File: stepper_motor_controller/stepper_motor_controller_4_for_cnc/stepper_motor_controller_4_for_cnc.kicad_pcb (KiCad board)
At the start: 2 copper layers, 31 parts, among them U1 74LS74, U11 LM317_TO-220, U3 74LS136

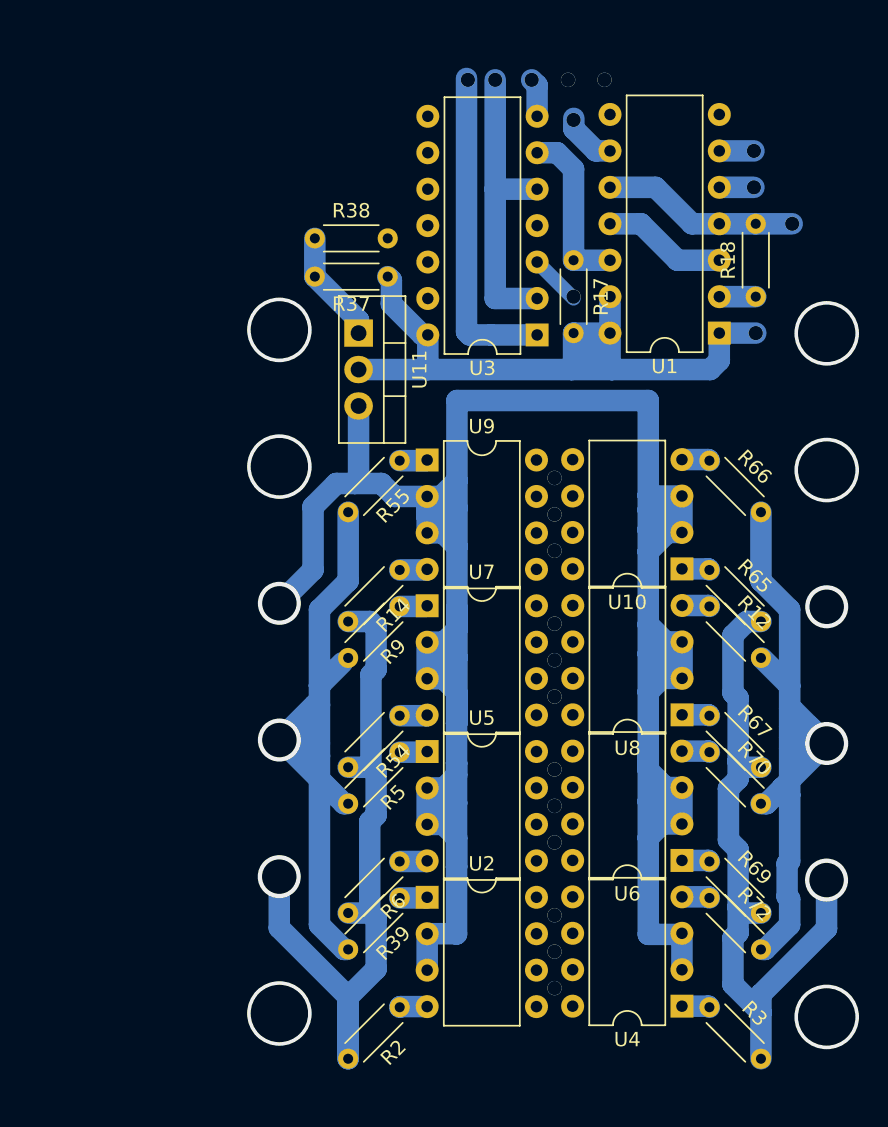
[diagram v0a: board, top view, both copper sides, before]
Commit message: move right
fdsaf
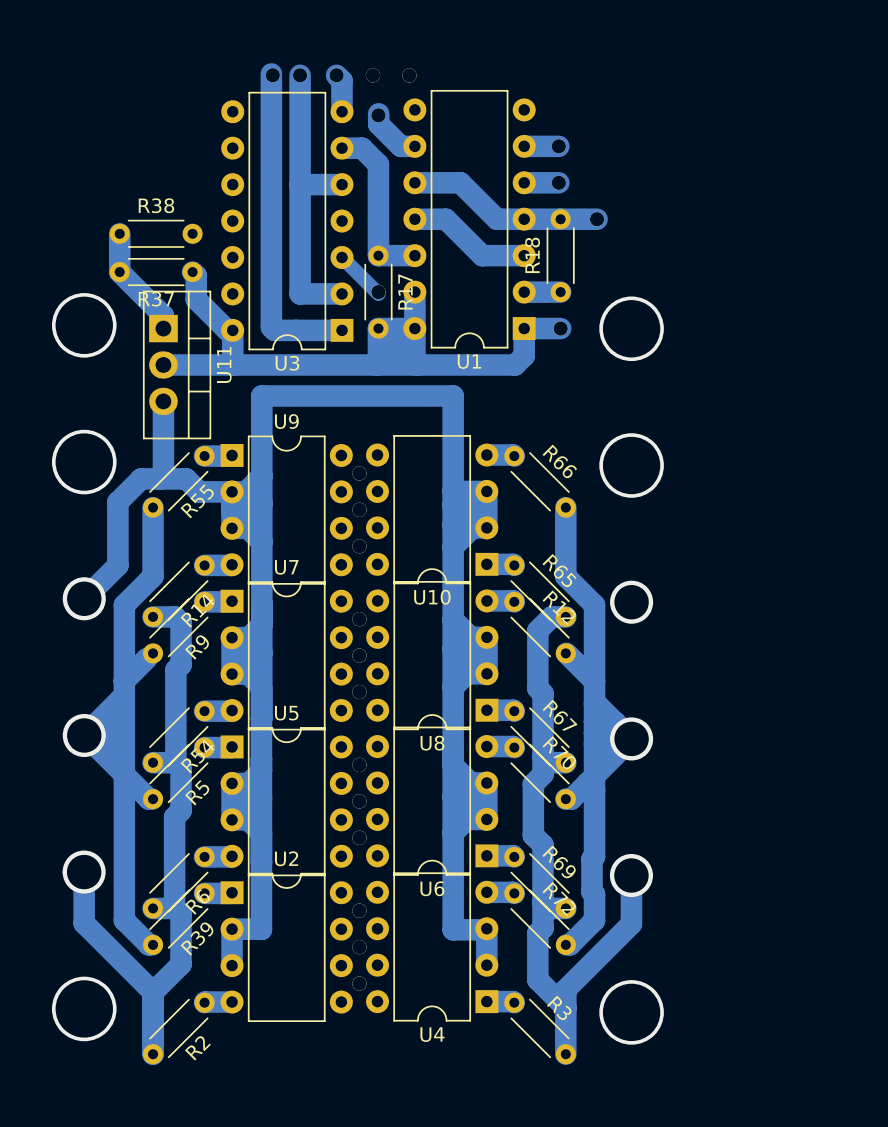
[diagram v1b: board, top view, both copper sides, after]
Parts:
- moved R12 13.6 mm to (35.5, -35.5)
- moved R17 13.6 mm to (26.0, -59.6)
- moved R3 13.6 mm to (35.5, -7.53)
- moved R65 13.6 mm to (35.5, -38.0)
- moved R66 13.6 mm to (35.5, -45.6)
- moved R67 13.6 mm to (35.5, -27.9)
- moved R69 13.6 mm to (35.5, -17.7)
- moved R70 13.6 mm to (35.5, -25.3)
- moved R72 13.6 mm to (35.5, -15.2)
- moved U10 13.6 mm to (33.6, -38.1)
- moved U3 13.6 mm to (23.5, -54.4)
- moved U4 13.6 mm to (33.6, -7.61)
- moved U6 13.6 mm to (33.6, -17.8)
- moved U8 13.6 mm to (33.6, -27.9)
- moved R14 13.6 mm to (13.9, -38.0)
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
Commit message: gerber
gerber
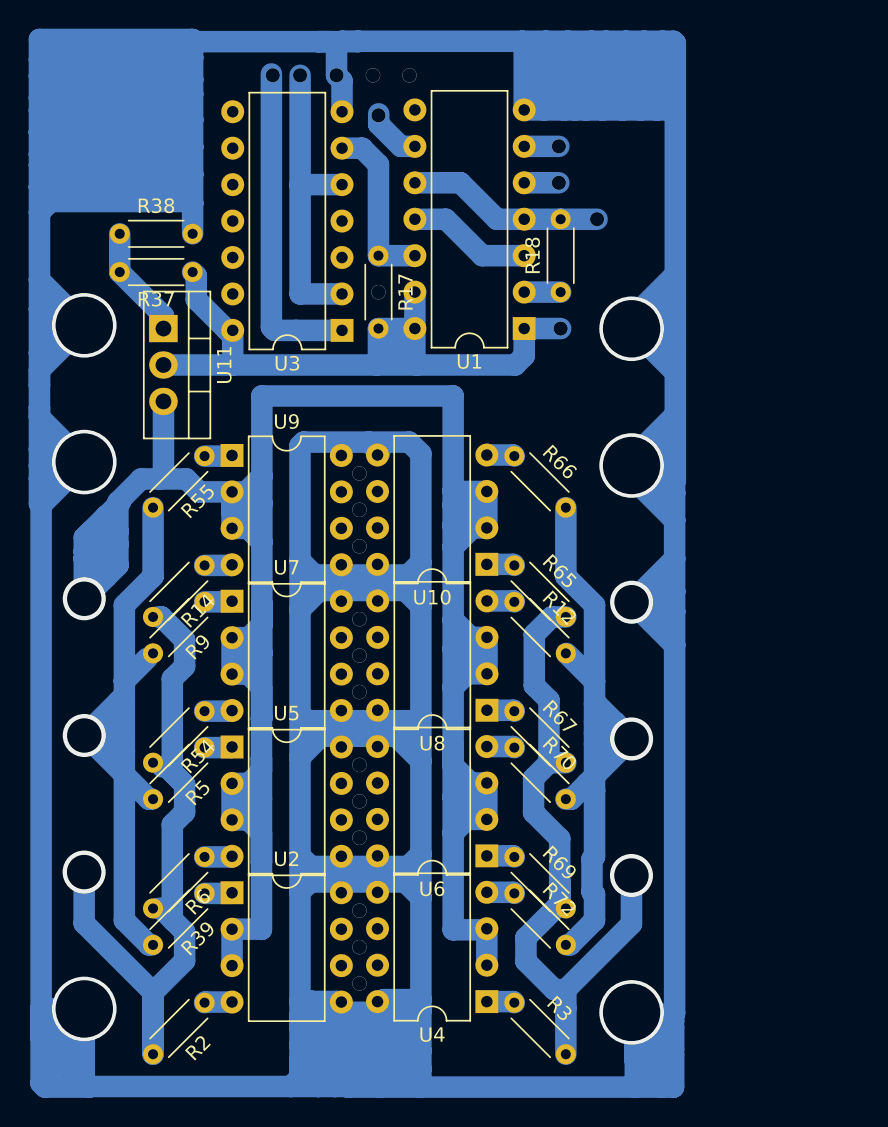
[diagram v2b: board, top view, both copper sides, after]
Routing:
- net GND: track 2.70 -> 803.9 mm
- net VCC: track 198.8 -> 216.2 mm
- net Net-(U1A-D): track 6.13 -> 2.55 mm
- net /C: track 48.2 -> 48.9 mm
